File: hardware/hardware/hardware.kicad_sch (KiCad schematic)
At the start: 18 parts, among them J1 RPi, J10 WaterLevel_01x05_Pin, J11 Conn_01x10_Pin, J12 Conn_01x10_Socket, J13 Moisture Sensor 4, J2 Conn_01x04_Socket, J3 Conn_01x04_Pin, J4 Rel_01x10_Pin, J5 ADC, J6 Moisture Sensor 1, J7 Moisture Sensor 2, J8 Moisture Sensor 3, J9 WaterLevel_01x05_Socket, U2 4010, U3 ULN2803A

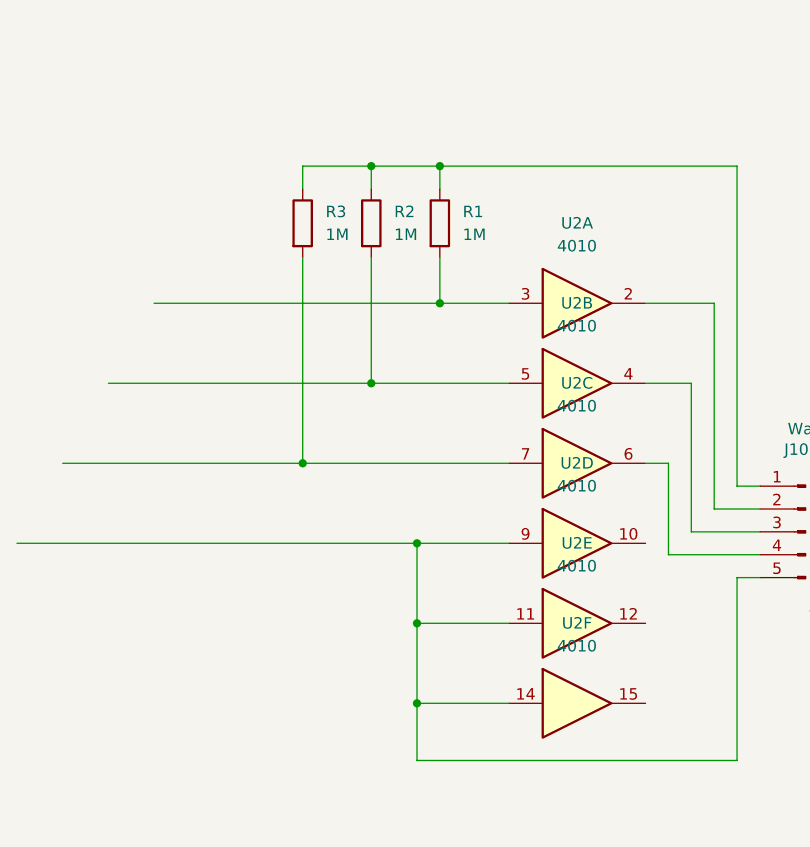
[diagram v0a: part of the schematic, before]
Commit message: updated schematic
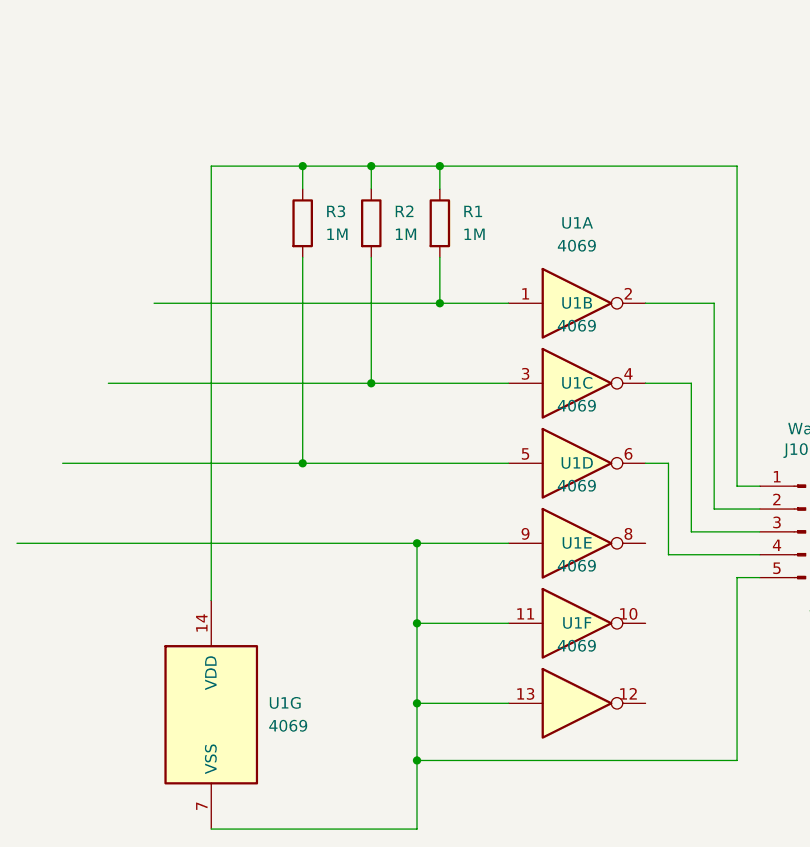
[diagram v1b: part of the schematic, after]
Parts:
- removed U2: 4010, symbol 4xxx:4010
- added U1: 4069, symbol 4xxx:4069
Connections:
- net at J10.1 (Pin_1), R1.1, R2.1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: now also U1.14 (VDD)
- net at R3.2: now also U1.5
- net at J10.3 (Pin_3): now also U1.4
- net at R2.2: now also U1.3
- net at J10.2 (Pin_2): now also U1.2
- net at R1.2: now also U1.1
- net at J10.5 (Pin_5): now also U1.11, U1.13, U1.7 (VSS), U1.9
- net at J10.4 (Pin_4): now also U1.6
